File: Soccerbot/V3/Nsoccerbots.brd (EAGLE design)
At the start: 149.8 x 101.3 mm, 64 parts, among them X1 NXT-SOCKET, X2 NXT-SOCKET, X3 NXT-SOCKET, X4 NXT-SOCKET

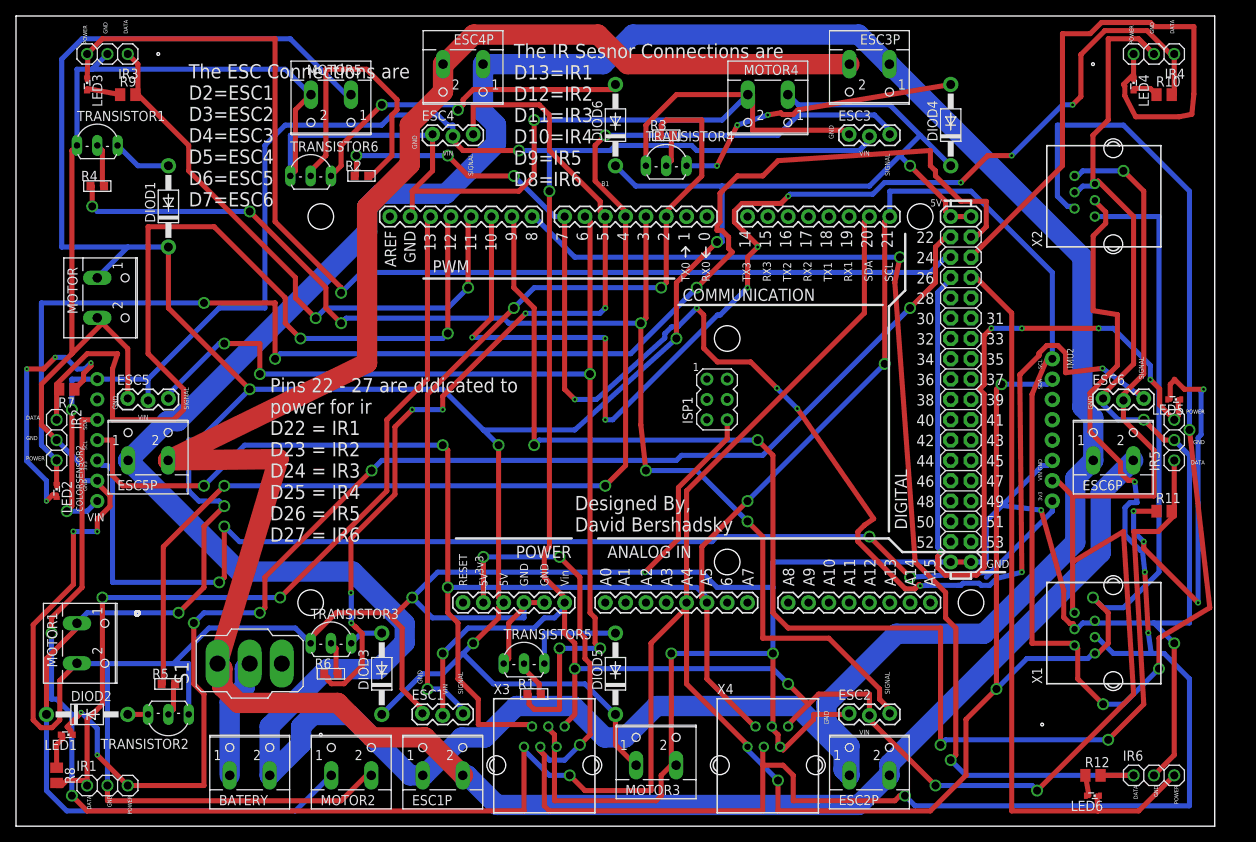
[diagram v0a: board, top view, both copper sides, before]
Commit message: S
s
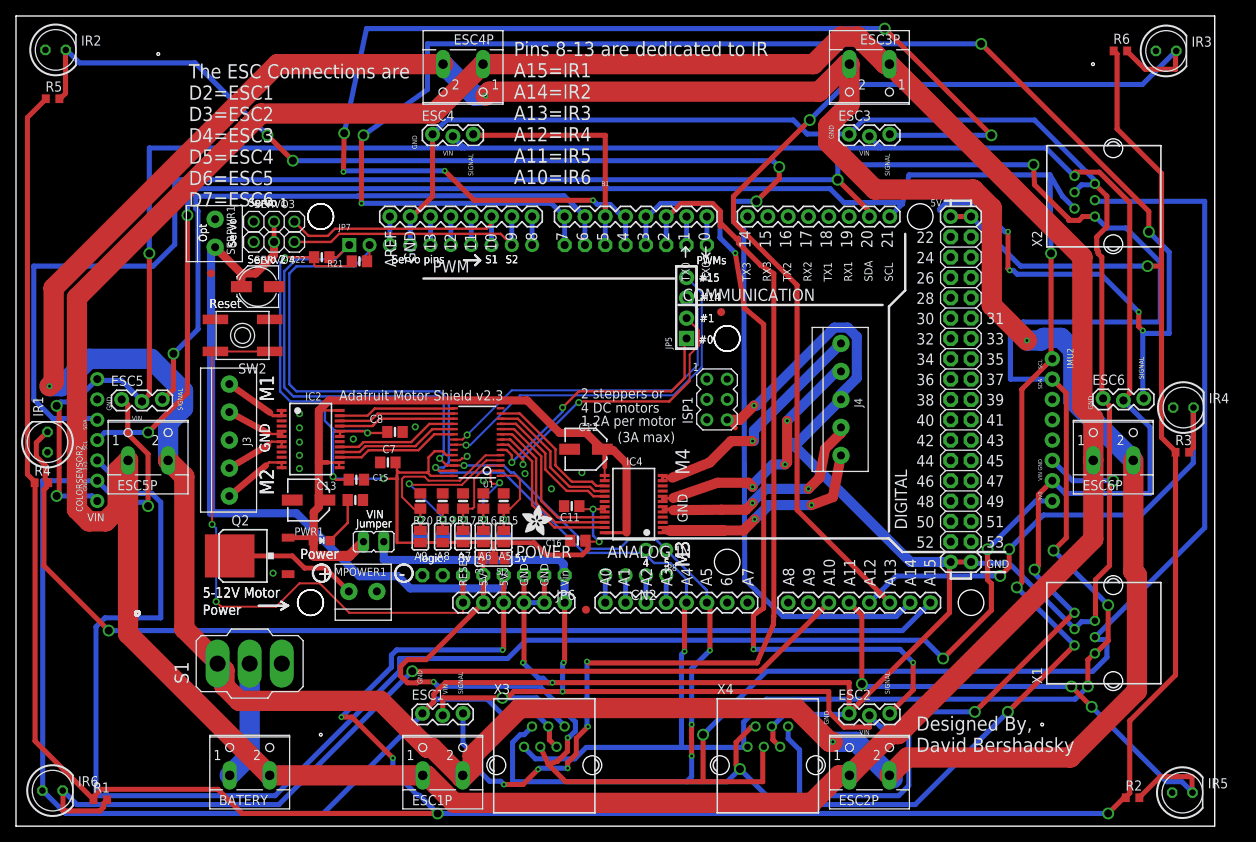
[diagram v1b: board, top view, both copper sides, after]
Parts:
- removed DIOD1, DIOD2, DIOD3, DIOD4, DIOD5, DIOD6: 1N4004, adafruit:DO41-10
- removed LED1, LED3, LED4, LED5, LED6: (no value), adafruit:SMARTLED-TTW
- removed MOTOR, MOTOR1, MOTOR2, MOTOR3, MOTOR4, MOTOR5: (no value), con-wago-500:W237-102
- removed R10, R11, R12, R7, R8, R9: (no value), adafruit:M0805
- removed TRANSISTOR1, TRANSISTOR2, TRANSISTOR3, TRANSISTOR4, TRANSISTOR5, TRANSISTOR6: 2N2907, adafruit:TO92-EBC-OVAL
- added A5, A6, A7, A8, A9: (no value), microbuilder:SOLDERJUMPER_REFLOW_NOPASTE
- added C11, C7, C8: 0.1uF, microbuilder:0805-NO
- added C12: 47uF/16v, microbuilder:PANASONIC_C
- added C13: 47uF+/16v, microbuilder:PANASONIC_C
- added C14: 10\0uF 6.3V, adafruit:PANASONIC_C
- added C15, C16: 10uF, microbuilder:0805-NO
- added CN2: 1X4-CLEANBIG, adafruit:1X04-CLEANBIG
- added D0-1, JP6: (no value), adafruit:1X08-CLEANBIG
- added IC2, IC4: TB6612FNG, adafruit:SSOP24
- added J3, J4: 1X5, adafruit:1X05-3.5MM
- added JP5: (no value), microbuilder:1X04_ROUND_76
- added JP7: (no value), microbuilder:1X10_ROUND70
- added JP8: (no value), microbuilder:1X02_ROUND
- added MPOWER1, SERPWR1: 1X2-3.5MM, adafruit:1X2-3.5MM
- added PWR1: (no value), jumper:JP1
- added Q2: AOD417, transistor-power:D-PAK_TO252AA
- added R15, R16, R17, R19, R20: 10k, microbuilder:0805-NO
- added R18: 1K, microbuilder:0805-NO
- added R21, R22: 10K, microbuilder:0805-NO
- added SERVO3, SERVO4: (no value), adafruit:1X03
- added SJ2: (no value), microbuilder:SOLDERJUMPER_2WAY_OPEN_NOPASTE
- added SW2: SPST_TACT-EVQQ2, adafruit:EVQ-Q2
- added TP10, TP6, TP7, TP8, TP9: (no value), microbuilder:TESTPOINT_ROUND_2MM
- added U$12, U$13, U$15: FIDUCIAL, adafruit:FIDUCIAL_1MM
- added U$17: (no value), microbuilder:ADAFRUIT_TEXT_30MM
- added U$18: (no value), microbuilder:ADAFRUIT_3.5MM
- added U1: PCA9685, microbuilder:TSSOP28
- IR1, IR2, IR3, IR4, IR5, IR6: device adafruit:1X03 -> led:LED5MM
- LED2: value (none) -> Green; device adafruit:SMARTLED-TTW -> microbuilder:CHIPLED_0805_NOOUTLINE
- R1, R2, R3, R4, R5, R6: device BaseApp:R0603 -> adafruit:R0603
- moved IR6 137.7 mm to (14.7, 3.17)
- moved IR3 132.3 mm to (153.9, 95.6), turned to 0 degrees
- moved R6 125.7 mm to (148.2, 95.6)
- moved R2 123.8 mm to (149.7, 2.29)
- moved R3 75.7 mm to (156.0, 45.5)
- moved R5 74.6 mm to (14.7, 89.7)
- moved R1 55.8 mm to (20.7, 2.03)
- moved IR2 48.8 mm to (15.1, 95.8), turned to 0 degrees
- moved IR4 44.3 mm to (156.1, 51.1), turned to 0 degrees
- moved IR5 44.1 mm to (156.0, 2.92), turned to 0 degrees
- moved IR1 43.6 mm to (14.1, 46.7), turned to 90 degrees
- moved R4 37.7 mm to (13.3, 41.7)
- moved LED2 33.7 mm to (48.4, 34.4), turned to 270 degrees
- moved ESC5 0.77 mm to (23.4, 51.9)
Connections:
- removed net N$10: DIOD5.A, TRANSISTOR5.C
- removed net N$11: DIOD4.A, TRANSISTOR4.C
- removed net N$12: R2.2, TRANSISTOR6.B
- removed net N$13: DIOD6.A, TRANSISTOR6.C
- removed net N$14: LED1.C@1, R8.1
- removed net N$15: LED2.C@1, R7.1
- removed net N$16: LED3.C@1, R9.1
- removed net N$17: LED4.C@1, R10.1
- removed net N$18: LED5.C@1, R11.1
- removed net N$19: LED6.C@1, R12.1
- removed net N$2: DIOD1.A, TRANSISTOR1.C
- removed net N$5: R5.2, TRANSISTOR2.B
- removed net N$6: DIOD2.A, TRANSISTOR2.C
- removed net N$7: R6.2, TRANSISTOR3.B
- removed net N$8: DIOD3.A, TRANSISTOR3.C
- removed net N$9: R1.2, TRANSISTOR5.B
- new net +12V: C12.+, C13.+, IC2.13, IC2.14, IC2.24, IC4.13, IC4.14, IC4.24, LED2.A, PWR1.1, Q2.3
- new net +5V: C14.+, SERPWR1.1, SERVO3.2, SERVO4.2, SJ2.1
- new net 18: A5.1, A6.1, A7.1, A8.2, A9.2, C11.1, C15.1, C16.1, C7.1, C8.1, IC2.19, IC2.20, IC4.19, IC4.20, R21.2, R22.2, SJ2.2, U1.24, U1.28
- new net 19: PWR1.2
- new net A4: A9.1, R20.2, TP6.P$1, U1.5
- new net GND1: IR5.A
- new net GND2: IR4.A
- new net GND3: IR1.A
- new net GND4: IR2.A
- new net GND5: IR3.A
- new net IOREF1: JP6.7
- new net M1A1: IC2.1, IC2.2, J3.5
- new net M1B1: IC2.5, IC2.6, J3.4
- new net M2A1: IC2.11, IC2.12, J3.1
- new net M2B1: IC2.7, IC2.8, J3.2
- new net M3A1: IC4.1, IC4.2, J4.1
- new net M3B1: IC4.5, IC4.6, J4.2
- new net M4A1: IC4.11, IC4.12, J4.5
- new net M4B1: IC4.7, IC4.8, J4.4
- new net PWM0: JP5.1, U1.6
- new net PWM1: JP5.2, U1.7
- new net PWM10: IC2.21, U1.17
- new net PWM11: IC2.17, U1.18
- new net PWM12: IC2.16, U1.19
- new net PWM13: IC2.15, U1.20
- new net PWM14: JP5.3, U1.21
- new net PWM15: JP5.4, U1.22
- new net PWM2: IC4.23, U1.8
- new net PWM3: IC4.22, U1.9
- new net PWM4: IC4.21, U1.10
- new net PWM5: IC4.17, U1.11
- new net PWM6: IC4.16, U1.12
- new net PWM7: IC4.15, U1.13
- new net PWM8: IC2.23, U1.15
- new net PWM9: IC2.22, U1.16
- new net VMOTOR1: MPOWER1.2, Q2.4
- net 3.3V: now also JP6.5, SJ2.3
- net 5.5V: now also JP6.4, R1.1, R2.1, R3.1, R4.1, R5.1, R6.1; no longer DIOD1.C, DIOD2.C, DIOD3.C, DIOD4.C, DIOD5.C, DIOD6.C, MOTOR.1, MOTOR1.1, MOTOR2.1, MOTOR3.1, MOTOR4.1, MOTOR5.1
- net A0: now also A5.2, CN2.4, R15.2, TP10.P$1, U1.1
- net A1: now also A6.2, CN2.3, R16.2, TP9.P$1, U1.2
- net A10: now also IR6.K, R1.2
- net A11: now also IR5.K, R2.2
- net A12: now also IR4.K, R3.2
- net A13: now also IR3.K, R6.2
- net A14: now also IR2.K, R5.2
- net A15: now also IR1.K, R4.2
- net A2: now also A7.2, CN2.2, R17.2, TP8.P$1, U1.3
- net A3: now also A8.1, CN2.1, R19.2, TP7.P$1, U1.4
- net AREF: now also JP7.3
- net D0: now also D0-1.1
- net D1: now also D0-1.2
- net D10: now also JP7.8, SERVO3.3; no longer IR4.1, R10.2
- net D11: now also JP7.7; no longer IR3.1, R9.2
- net D12: now also JP7.6; no longer IR2.1, R7.2
- net D13: now also JP7.5; no longer IR1.1, R8.2
- net D2: now also D0-1.3; no longer R3.1
- net D22: no longer IR1.3, LED1.A@1
- net D23: no longer IR2.3, LED2.A@1
- net D24: no longer IR3.3, LED3.A@1
- net D25: no longer IR4.3, LED4.A@1
- net D26: no longer IR5.3, LED5.A@1
- net D27: no longer IR6.3, LED6.A@1
- net D3: now also D0-1.4; no longer R4.1
- net D4: now also D0-1.5; no longer R5.1
- net D5: now also D0-1.6; no longer R6.1
- net D6: now also D0-1.7; no longer R1.1
- net D7: now also D0-1.8; no longer R2.1
- net D8: now also JP7.10; no longer IR6.1, R12.2
- net D9: now also JP7.9, SERVO4.3; no longer IR5.1, R11.2
- net GND: now also C11.2, C12.-, C13.-, C14.-, C15.2, C16.2, C7.2, C8.2, IC2.10, IC2.18, IC2.3, IC2.4, IC2.9, IC4.10, IC4.18, IC4.3, IC4.4, IC4.9, IR6.A, J3.3, J4.3, JP6.2, JP6.3, JP7.4, MPOWER1.1, Q2.1, R15.1, R16.1, R17.1, R18.1, R19.1, R20.1, SERPWR1.2, SERVO3.1, SERVO4.1, SW2.A, SW2.A', U1.14, U1.23, U1.25; no longer IR1.2, IR2.2, IR3.2, IR4.2, IR5.2, IR6.2, MOTOR.2, MOTOR1.2, MOTOR2.2, MOTOR3.2, MOTOR4.2, MOTOR5.2, TRANSISTOR1.E, TRANSISTOR2.E, TRANSISTOR3.E, TRANSISTOR4.E, TRANSISTOR5.E, TRANSISTOR6.E
- net N$1: now also LED2.C, R18.2; no longer R4.2, TRANSISTOR1.B
- net N$3: now also JP6.8; no longer R3.2, TRANSISTOR4.B
- net RESET: now also JP6.6, SW2.B, SW2.B'
- net SCL: now also JP7.1, JP8.1, R22.1, U1.26
- net SDA: now also JP7.2, JP8.2, R21.1, U1.27
- net VIN: now also JP6.1
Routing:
- net GND: track 795.2 -> 524.7 mm, vias 10 -> 19
- net A14: track 0.00 -> 181.4 mm, vias 0 -> 4
- net D23: track 176.0 -> 0.00 mm, vias 3 -> 0
- net D22: track 165.1 -> 0.00 mm, vias 6 -> 0
- net D9: track 179.1 -> 31.7 mm, vias 4 -> 0
- net D24: track 140.9 -> 0.00 mm, vias 1 -> 0
- net D8: track 141.2 -> 3.56 mm, vias 2 -> 0
- net 18: track 0.00 -> 137.1 mm, vias 0 -> 6
- net A15: track 0.00 -> 133.8 mm, vias 0 -> 1
- net A13: track 0.00 -> 131.1 mm, vias 0 -> 1
- net D10: track 152.9 -> 32.2 mm, vias 9 -> 0
- net A10: track 0.00 -> 115.9 mm, vias 0 -> 1
- net BAT+: track 309.6 -> 424.9 mm, vias 0 -> 4
- net D12: track 116.8 -> 3.56 mm, vias 2 -> 0
- net D26: track 107.2 -> 0.00 mm, vias 5 -> 0
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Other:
- board text added: "#0"
- board text added: "#1"
- board text added: "#14"
- board text added: "#15"
- board text added: "(3A max)"
- board text added: "+"
- board text added: "-"
- board text added: "1.2A per motor"
- board text added: "2 steppers or"
- board text added: "3v"
- board text added: "4"
- board text added: "4 DC motors"
- board text added: "5"
- board text added: "5-12V Motor"
- board text added: "5v"
- board text added: "Adafruit Motor Shield v2! Control 4 DC Motors or 2 Stepper motors via I2C Pins used: SDA, SCL & A4 tied to SDA, A5 to SCL"
- board text added: "Adafruit Motor Shield v2.3"
- board text added: "For opt. servo"
- board text added: "Jumper"
- board text added: "M1"
- board text added: "M2"
- board text added: "M3"
- board text added: "M4"
- board text added: "Opt"
- board text added: "PWMs"
- board text added: "Pins 8-13 are dedicated to IR A15=IR1 A14=IR2 A13=IR3 A12=IR4 A11=IR5 A10=IR6"
- board text added: "Power"
- board text added: "Reset"
- board text added: "S1"
- board text added: "S2"
- board text added: "Servo"
- board text added: "Servo 1"
- board text added: "Servo 2"
- board text added: "Servo pins"
- board text added: "logic:"
- board text added: "pwr supply cut trace"
- board text removed: "DATA"
- board text removed: "POWER"
- board text removed: "Pins 22 - 27 are didicated to power for ir D22 = IR1 D23 = IR2 D24 = IR3 D25 = IR4 D26 = IR5 D27 = IR6"
- board text removed: "The IR Sesnor Connections are D13=IR1 D12=IR2 D11=IR3 D10=IR4 D9=IR5 D8=IR6"
